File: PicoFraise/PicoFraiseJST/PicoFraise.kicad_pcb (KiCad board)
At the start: 2 copper layers, 49.5 x 49.5 mm, 21 parts, among them J1 Conn_01x06, J2 Conn_01x06, J3 Conn_01x06, J4 Conn_01x06, J5 Conn_01x06, J6 Conn_01x06, J7 Reset, J8 12-24V input, U1 Pico, U2 L7805

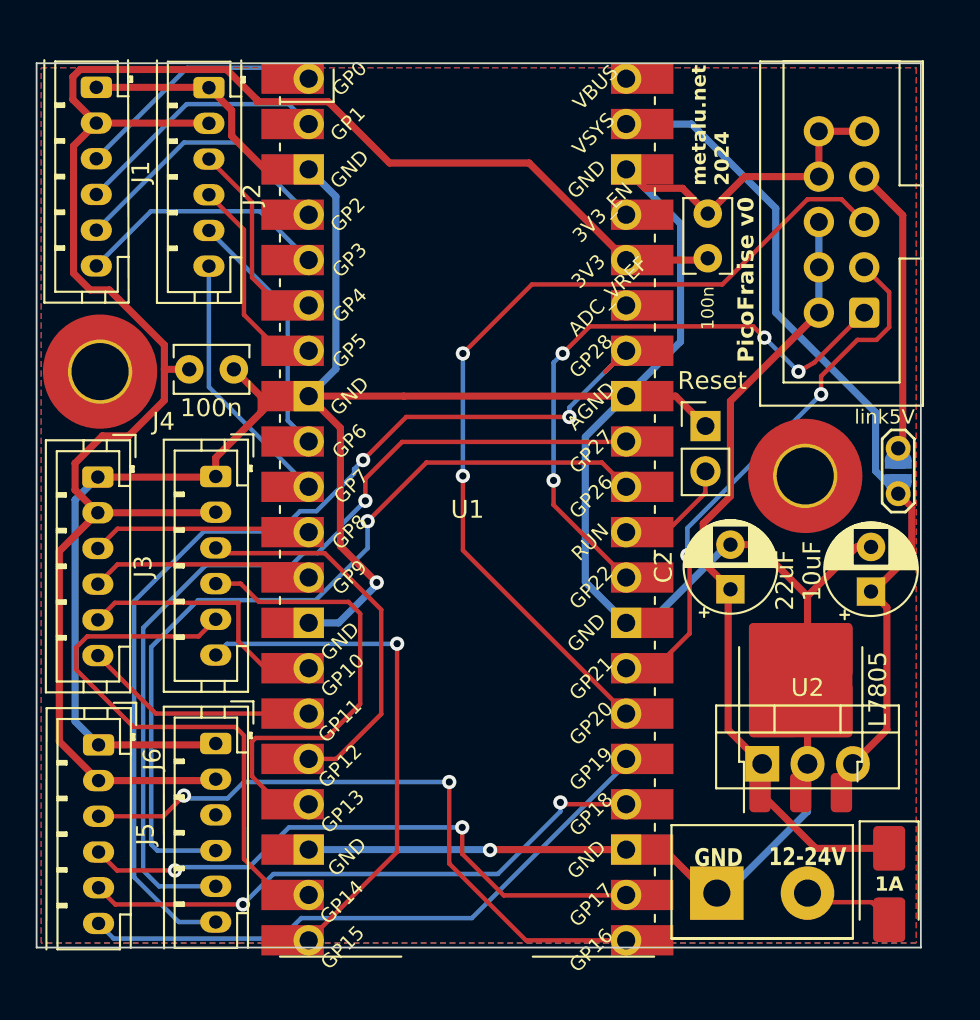
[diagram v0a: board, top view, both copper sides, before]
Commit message: update PicoFraiseJST
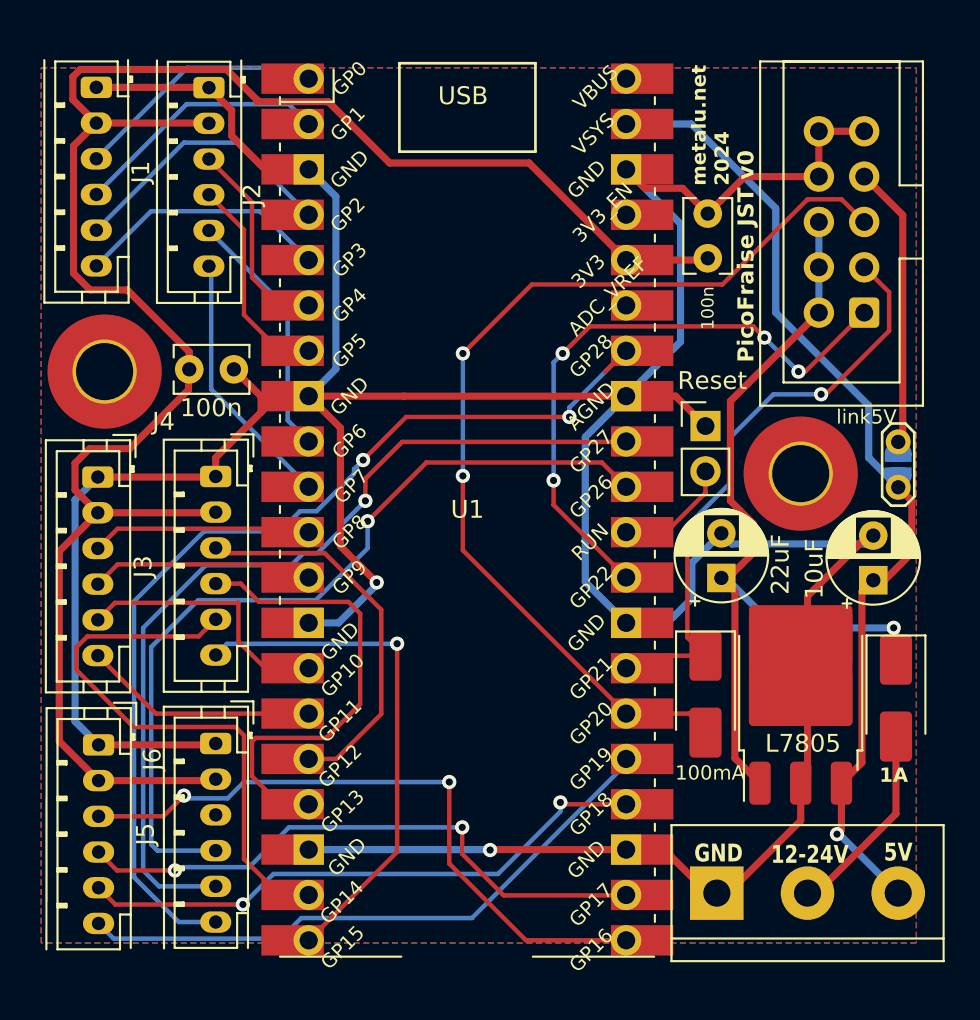
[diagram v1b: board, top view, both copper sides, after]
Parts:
- removed U2: L7805, Package_TO_SOT_THT:TO-220-3_Vertical
- added D2: 100mA, Diode_SMD:D_SMA, F.Cu at (151.8, 98.8)
- J8: footprint TerminalBlock:TerminalBlock_bornier-2_P5.08mm -> TerminalBlock:TerminalBlock_bornier-3_P5.08mm
- moved D1 10.4 mm to (162.4, 99.1)
- moved C2 0.81 mm to (152.7, 92.3)
- moved C3 0.65 mm to (161.2, 92.5)
- moved Ubis2 0.63 mm to (157.1, 98.7)
- moved JP1 0.38 mm to (162.6, 86.0)
- moved JP2 0.36 mm to (162.6, 87.2)
- moved H2 0.28 mm to (157.1, 86.5)
- moved H1 0.25 mm to (118.1, 80.8)
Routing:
- net +5V: track 46.8 -> 56.3 mm, vias 0 -> 1
- net Net-(D1-A): track 5.19 -> 11.8 mm
- net +12V: track 42.5 -> 48.5 mm, vias 0 -> 1
- net GND: track 218.2 -> 223.0 mm
- net /RX: track 50.5 -> 55.4 mm
- net /TX: track 30.8 -> 34.0 mm
- net +3.3V: track 109.7 -> 110.5 mm
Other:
- board outline removed
- board text added: "PicoFraise JST v0"
- board text added: "USB"
- board text removed: "PicoFraise v0"
